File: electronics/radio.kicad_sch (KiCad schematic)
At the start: 30 parts, among them J7 SIM_Card, J9 Conn_Coaxial_Small, Q1 Q_NMOS_GSD, SW1 SW_Push, U2 TPS22953

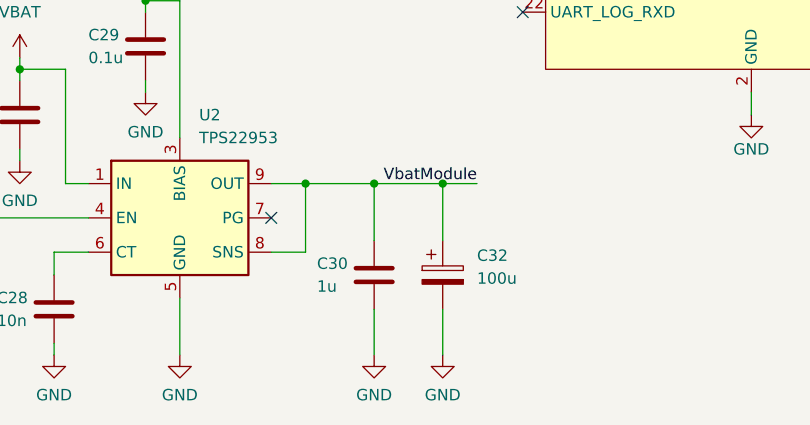
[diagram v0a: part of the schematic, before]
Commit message: electronics: initial placement
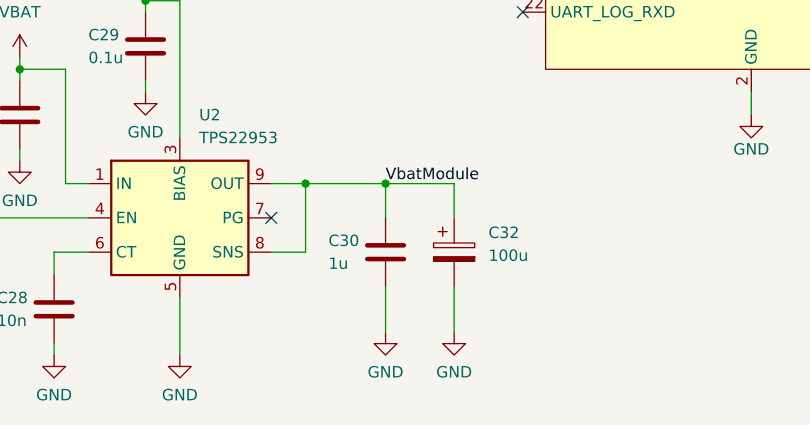
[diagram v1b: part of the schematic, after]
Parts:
- Q1: footprint (none) -> Package_TO_SOT_SMD:SOT-23-3
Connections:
- net VBAT: no longer C24.1, C25.1, C26.1, C30.1, C32.1, C8.1, R26.1, U2.10 (OUT), U2.8 (SNS), U2.9 (OUT), U4.55 (VBAT), U4.56 (VBAT), U4.57 (VBAT)
- new net VbatModule: C24.1, C25.1, C26.1, C30.1, C32.1, C8.1, R26.1, U2.10 (OUT), U2.8 (SNS), U2.9 (OUT), U4.55 (VBAT), U4.56 (VBAT), U4.57 (VBAT)
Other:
- moved on the sheet: C30, C32
